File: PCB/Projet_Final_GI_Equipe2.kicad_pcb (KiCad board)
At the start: 2 copper layers, 104.8 x 99.1 mm, 30 parts, among them J1 Conn_01x15_Female, J2 Conn_01x15_Female, J3 mcp2gauche, J4 mcp1gauche, J5 mcp1droite, J6 mcp2droite, J7 Conn_01x03_Male, J8 Conn_01x02_Male, SW1 SW_Push, SW2 SW_Push, U1 COM-09032, U2 COM-09032, U3 AZ1117-5.0

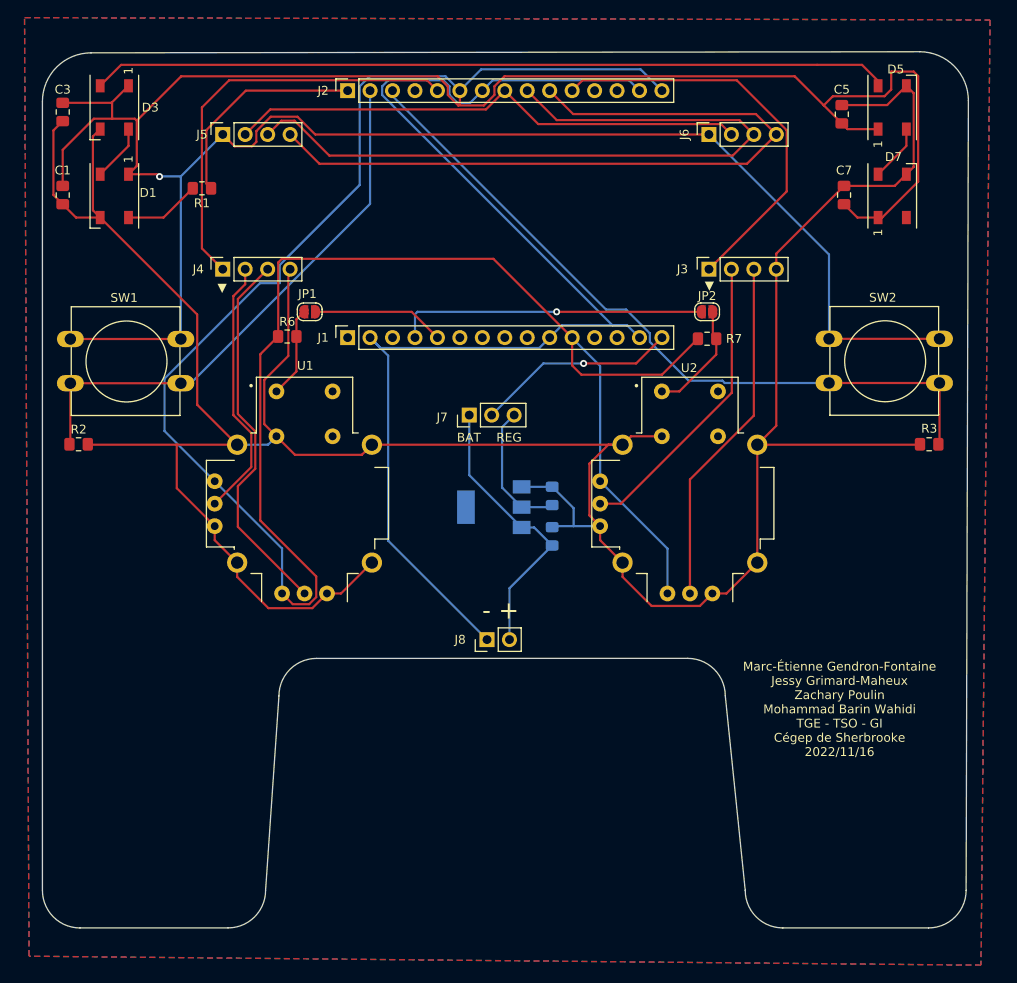
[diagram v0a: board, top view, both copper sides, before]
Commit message: Version final PCB Zachary
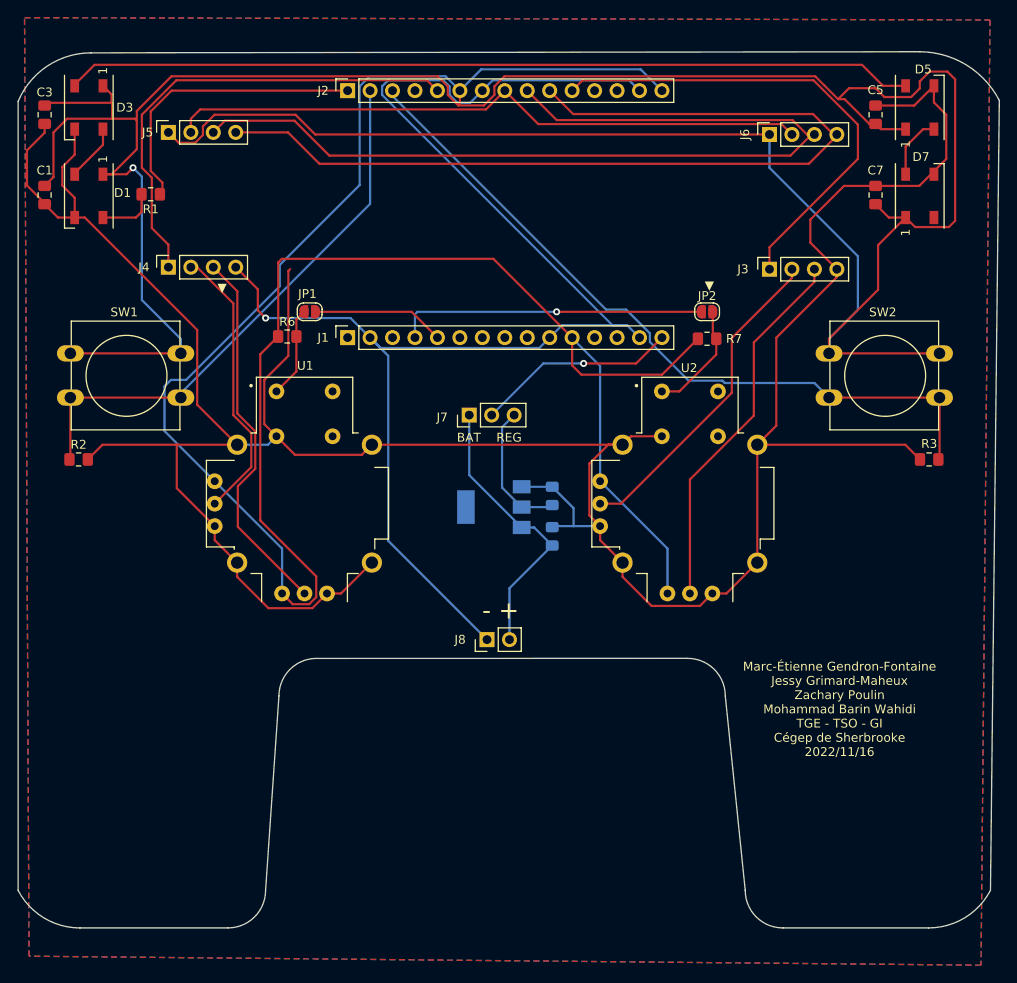
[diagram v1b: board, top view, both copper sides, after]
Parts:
- moved J3 6.85 mm to (178.0, 77.5)
- moved J6 6.85 mm to (178.0, 62.2)
- moved J5 6.15 mm to (110.0, 62.0)
- moved J4 6.15 mm to (110.0, 77.2)
- moved R1 5.83 mm to (108.0, 69.0)
- moved C5 3.82 mm to (190.0, 60.0)
- moved C7 3.56 mm to (190.0, 69.1)
- moved D5 3.11 mm to (195.0, 59.2)
- moved D7 3.11 mm to (195.0, 69.2)
- moved D1 2.89 mm to (101.0, 69.2)
- moved D3 2.89 mm to (101.0, 59.2)
- moved C3 2.07 mm to (96.0, 60.0)
- moved C1 2.04 mm to (96.0, 69.1)
- moved R2 1.72 mm to (99.8, 99.0)
- moved R3 1.72 mm to (196.1, 99.0)
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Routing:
- net /3.3V: track 550.9 -> 595.9 mm
- net GND: track 470.3 -> 498.9 mm, vias 0 -> 1
- net /D7/DIN: track 85.4 -> 105.5 mm
- net /D6/DOUT: track 86.0 -> 105.7 mm
- net /D5/CLK: track 59.1 -> 72.9 mm
- net /D8/CSR: track 46.5 -> 55.4 mm
- net /D0/RGB: track 24.6 -> 33.3 mm
- net /D4/CSL: track 47.7 -> 54.0 mm
- net Net-(D3-Pad2): track 90.3 -> 96.0 mm
- net /RIGHTH: track 39.7 -> 42.5 mm
- net /RIGHTV: track 34.1 -> 36.9 mm
- net /LEFTV: track 29.6 -> 31.7 mm
- net Net-(D1-Pad4): track 8.64 -> 6.62 mm
- net /D1/ATTACK: track 62.1 -> 63.1 mm
- net /D2/SPECIAL: track 83.5 -> 84.2 mm
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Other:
- board size 104.8 x 99.1 mm -> 111 x 99.1 mm
